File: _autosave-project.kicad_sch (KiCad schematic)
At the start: 160 parts, among them SW1 SW_Push, U1 ATmega32U4-A, Y1 16MHz

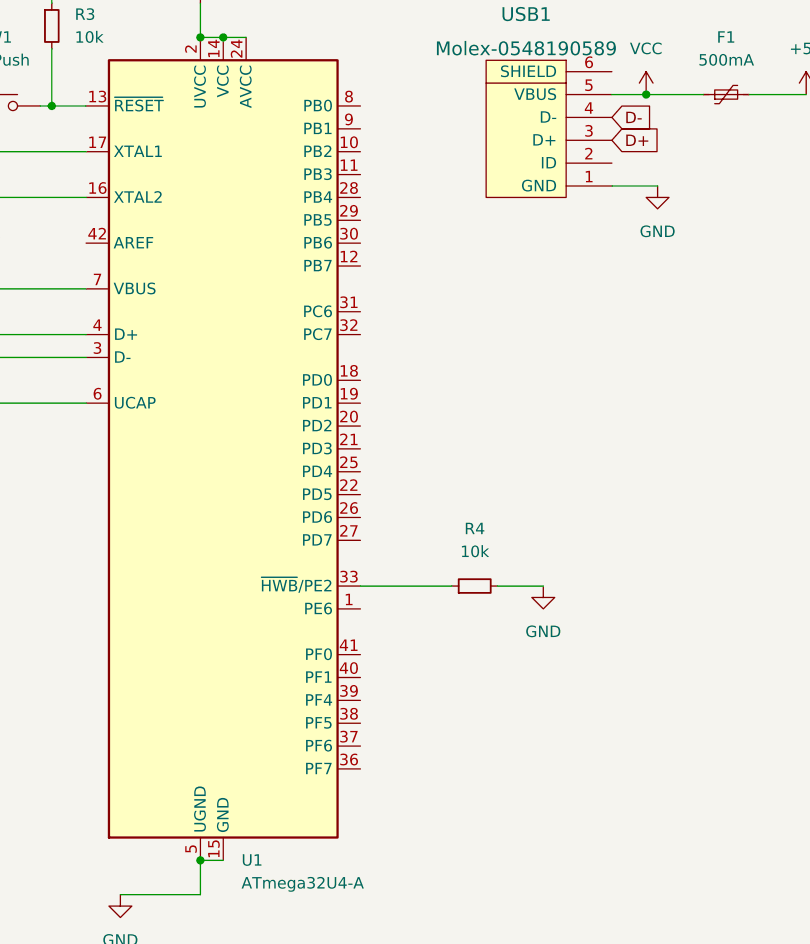
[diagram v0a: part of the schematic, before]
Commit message: kind of done? no checks or fills
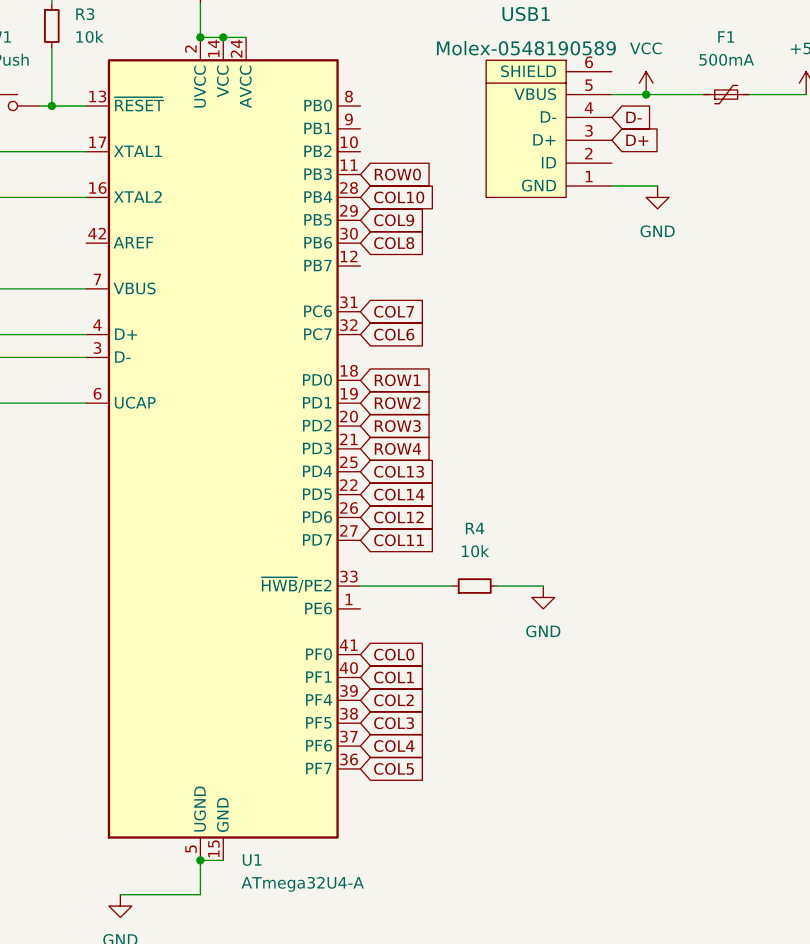
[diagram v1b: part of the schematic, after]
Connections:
- net COL0: now also U1.41 (PF0)
- net COL1: now also U1.40 (PF1)
- net COL10: now also U1.28 (PB4)
- net COL11: now also U1.27 (PD7)
- net COL12: now also U1.26 (PD6)
- net COL13: now also U1.25 (PD4)
- net COL14: now also U1.22 (PD5)
- net COL2: now also U1.39 (PF4)
- net COL3: now also U1.38 (PF5)
- net COL4: now also U1.37 (PF6)
- net COL5: now also U1.36 (PF7)
- net COL6: now also U1.32 (PC7)
- net COL7: now also U1.31 (PC6)
- net COL8: now also U1.30 (PB6)
- net COL9: now also U1.29 (PB5)
- net ROW0: now also U1.11 (PB3)
- net ROW1: now also U1.18 (PD0)
- net ROW2: now also U1.19 (PD1)
- net ROW3: now also U1.20 (PD2)
- net ROW4: now also U1.21 (PD3)
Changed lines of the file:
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@@
+    )
+  )
+  (global_label "COL14" (shape input) (at 105.41 92.71 0) (fields_autoplaced)
+    (effects (font (size 1.27 1.27)) (justify left))
+    (property "Intersheet References" "${INTERSHEET_REFS}" (id 0) (at 113.8707 92.6306 0)
+      (effects (font (size 1.27 1.27)) (justify left) hide)
     )
   )
@@
     )
   )
+  (global_label "ROW0" (shape input) (at 105.41 57.15 0) (fields_autoplaced)
+    (effects (font (size 1.27 1.27)) (justify left))
+    (property "Intersheet References" "${INTERSHEET_REFS}" (id 0) (at 113.0845 57.0706 0)
+      (effects (font (size 1.27 1.27)) (justify left) hide)
+    )
+  )
+  (global_label "COL12" (shape input) (at 105.41 95.25 0) (fields_autoplaced)
+    (effects (font (size 1.27 1.27)) (justify left))
+    (property "Intersheet References" "${INTERSHEET_REFS}" (id 0) (at 113.8707 95.1706 0)
+      (effects (font (size 1.27 1.27)) (justify left) hide)
+    )
+  )
   (global_label "ROW4" (shape input) (at 163.83 113.03 180) (fields_autoplaced)
     (effects (font (size 1.27 1.27)) (justify right))
@@
     )
   )
+  (global_label "COL11" (shape input) (at 105.41 97.79 0) (fields_autoplaced)
+    (effects (font (size 1.27 1.27)) (justify left))
+    (property "Intersheet References" "${INTERSHEET_REFS}" (id 0) (at 113.8707 97.7106 0)
+      (effects (font (size 1.27 1.27)) (justify left) hide)
+    )
+  )
+  (global_label "COL8" (shape input) (at 105.41 64.77 0) (fields_autoplaced)
+    (effects (font (size 1.27 1.27)) (justify left))
+    (property "Intersheet References" "${INTERSHEET_REFS}" (id 0) (at 112.6612 64.6906 0)
+      (effects (font (size 1.27 1.27)) (justify left) hide)
+    )
+  )
   (global_label "COL10" (shape input) (at 283.21 31.75 90) (fields_autoplaced)
     (effects (font (size 1.27 1.27)) (justify left))
@@
     )
   )
+  (global_label "COL6" (shape input) (at 105.41 74.93 0) (fields_autoplaced)
+    (effects (font (size 1.27 1.27)) (justify left))
+    (property "Intersheet References" "${INTERSHEET_REFS}" (id 0) (at 112.6612 74.8506 0)
+      (effects (font (size 1.27 1.27)) (justify left) hide)
+    )
+  )
+  (global_label "COL3" (shape input) (at 105.41 118.11 0) (fields_autoplaced)
+    (effects (font (size 1.27 1.27)) (justify left))
+    (property "Intersheet References" "${INTERSHEET_REFS}" (id 0) (at 112.6612 118.0306 0)
+      (effects (font (size 1.27 1.27)) (justify left) hide)
+    )
+  )
   (global_label "COL5" (shape input) (at 232.41 30.48 90) (fields_autoplaced)
     (effects (font (size 1.27 1.27)) (justify left))
@@
     )
   )
+  (global_label "COL7" (shape input) (at 105.41 72.39 0) (fields_autoplaced)
+    (effects (font (size 1.27 1.27)) (justify left))
+    (property "Intersheet References" "${INTERSHEET_REFS}" (id 0) (at 112.6612 72.3106 0)
+      (effects (font (size 1.27 1.27)) (justify left) hide)
+    )
+  )
   (global_label "COL14" (shape input) (at 323.85 31.75 90) (fields_autoplaced)
     (effects (font (size 1.27 1.27)) (justify left))
@@
     )
   )
+  (global_label "ROW1" (shape input) (at 105.41 80.01 0) (fields_autoplaced)
+    (effects (font (size 1.27 1.27)) (justify left))
+    (property "Intersheet References" "${INTERSHEET_REFS}" (id 0) (at 113.0845 79.9306 0)
+      (effects (font (size 1.27 1.27)) (justify left) hide)
+    )
+  )
+  (global_label "COL0" (shape input) (at 105.41 110.49 0) (fields_autoplaced)
+    (effects (font (size 1.27 1.27)) (justify left))
+    (property "Intersheet References" "${INTERSHEET_REFS}" (id 0) (at 112.6612 110.4106 0)
+      (effects (font (size 1.27 1.27)) (justify left) hide)
+    )
+  )
+  (global_label "COL13" (shape input) (at 105.41 90.17 0) (fields_autoplaced)
+    (effects (font (size 1.27 1.27)) (justify left))
+    (property "Intersheet References" "${INTERSHEET_REFS}" (id 0) (at 113.8707 90.0906 0)
+      (effects (font (size 1.27 1.27)) (justify left) hide)
+    )
+  )
+  (global_label "COL9" (shape input) (at 105.41 62.23 0) (fields_autoplaced)
+    (effects (font (size 1.27 1.27)) (justify left))
+    (property "Intersheet References" "${INTERSHEET_REFS}" (id 0) (at 112.6612 62.1506 0)
+      (effects (font (size 1.27 1.27)) (justify left) hide)
+    )
+  )
   (global_label "COL12" (shape input) (at 303.53 31.75 90) (fields_autoplaced)
     (effects (font (size 1.27 1.27)) (justify left))
@@
     )
   )
+  (global_label "ROW2" (shape input) (at 105.41 82.55 0) (fields_autoplaced)
+    (effects (font (size 1.27 1.27)) (justify left))
+    (property "Intersheet References" "${INTERSHEET_REFS}" (id 0) (at 113.0845 82.4706 0)
+      (effects (font (size 1.27 1.27)) (justify left) hide)
+    )
+  )
   (global_label "COL3" (shape input) (at 212.09 30.48 90) (fields_autoplaced)
     (effects (font (size 1.27 1.27)) (justify left))
@@
     )
   )
+  (global_label "COL1" (shape input) (at 105.41 113.03 0) (fields_autoplaced)
+    (effects (font (size 1.27 1.27)) (justify left))
+    (property "Intersheet References" "${INTERSHEET_REFS}" (id 0) (at 112.6612 112.9506 0)
+      (effects (font (size 1.27 1.27)) (justify left) hide)
+    )
+  )
   (global_label "D+" (shape input) (at 133.35 53.34 0) (fields_autoplaced)
     (effects (font (size 1.27 1.27)) (justify left))
@@
     )
   )
+  (global_label "COL2" (shape input) (at 105.41 115.57 0) (fields_autoplaced)
+    (effects (font (size 1.27 1.27)) (justify left))
+    (property "Intersheet References" "${INTERSHEET_REFS}" (id 0) (at 112.6612 115.4906 0)
+      (effects (font (size 1.27 1.27)) (justify left) hide)
+    )
+  )
   (global_label "COL1" (shape input) (at 191.77 30.48 90) (fields_autoplaced)
     (effects (font (size 1.27 1.27)) (justify left))
@@
     )
   )
+  (global_label "ROW4" (shape input) (at 105.41 87.63 0) (fields_autoplaced)
+    (effects (font (size 1.27 1.27)) (justify left))
+    (property "Intersheet References" "${INTERSHEET_REFS}" (id 0) (at 113.0845 87.5506 0)
+      (effects (font (size 1.27 1.27)) (justify left) hide)
+    )
+  )
   (global_label "D-" (shape input) (at 35.56 77.47 180) (fields_autoplaced)
     (effects (font (size 1.27 1.27)) (justify right))
@@
       (effects (font (size 1.27 1.27)) (justify left) hide)
     )
+  )
+  (global_label "ROW3" (shape input) (at 105.41 85.09 0) (fields_autoplaced)
+    (effects (font (size 1.27 1.27)) (justify left))
+    (property "Intersheet References" "${INTERSHEET_REFS}" (id 0) (at 113.0845 85.0106 0)
+      (effects (font (size 1.27 1.27)) (justify left) hide)
+    )
+  )
+  (global_label "COL4" (shape input) (at 105.41 120.65 0) (fields_autoplaced)
+    (effects (font (size 1.27 1.27)) (justify left))
+    (property "Intersheet References" "${INTERSHEET_REFS}" (id 0) (at 112.6612 120.5706 0)
+      (effects (font (size 1.27 1.27)) (justify left) hide)
+    )
+  )
+  (global_label "COL10" (shape input) (at 105.41 59.69 0) (fields_autoplaced)
+    (effects (font (size 1.27 1.27)) (justify left))
+    (property "Intersheet References" "${INTERSHEET_REFS}" (id 0) (at 113.8707 59.6106 0)
+      (effects (font (size 1.27 1.27)) (justify left) hide)
+    )
+  )
+  (global_label "COL5" (shape input) (at 105.41 123.19 0) (fields_autoplaced)
+    (effects (font (size 1.27 1.27)) (justify left))
+    (property "Intersheet References" "${INTERSHEET_REFS}" (id 0) (at 112.6612 123.1106 0)
+      (effects (font (size 1.27 1.27)) (justify left) hide)
+    )
